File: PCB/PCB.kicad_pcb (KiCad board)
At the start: 4 copper layers, 21 x 51 mm, 33 parts, among them J1 USB_C_Receptacle_USB2.0_16P, J2 Conn_01x20, J3 Conn_01x20, SW1 SW_Push, U1 RP2040, U2 MCP1700x-330xxTT, U3 W25Q128JVS, Y1 Crystal_GND24

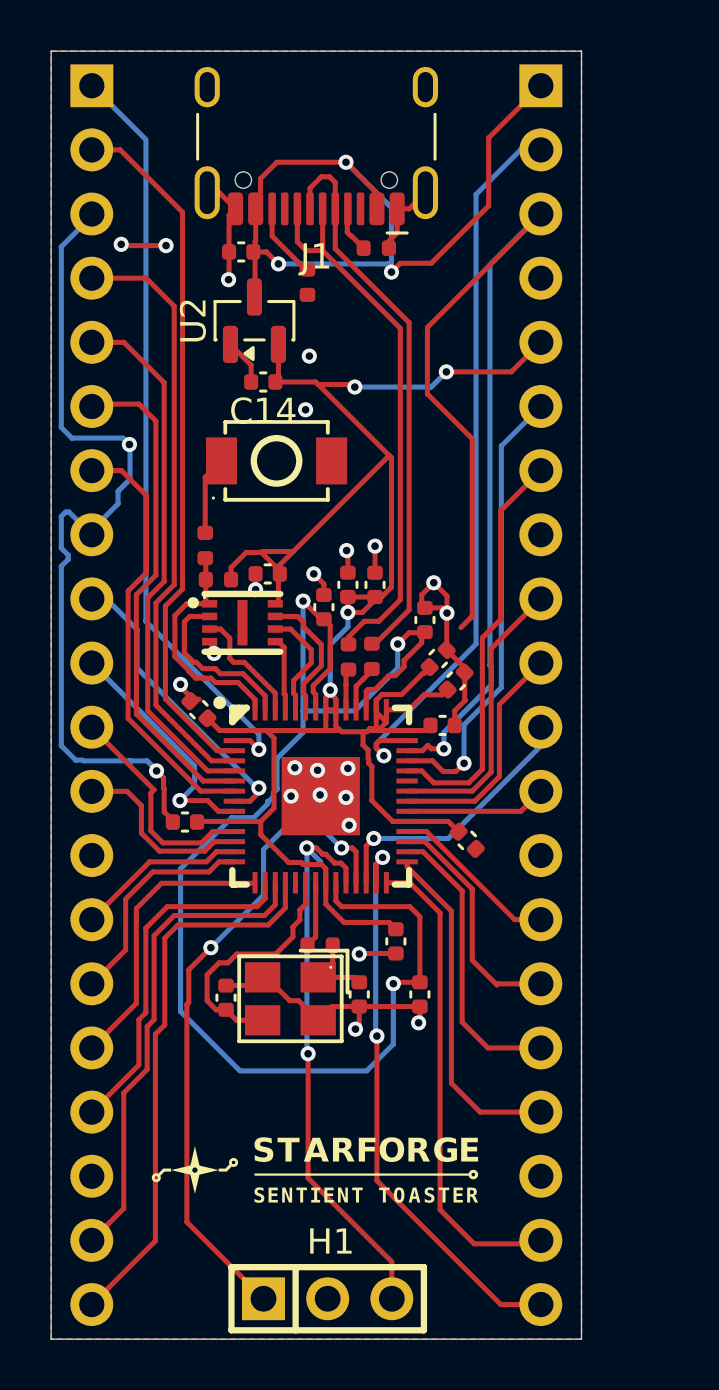
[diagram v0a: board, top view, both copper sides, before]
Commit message: finishing up project with BOM and FAB complete and clean.
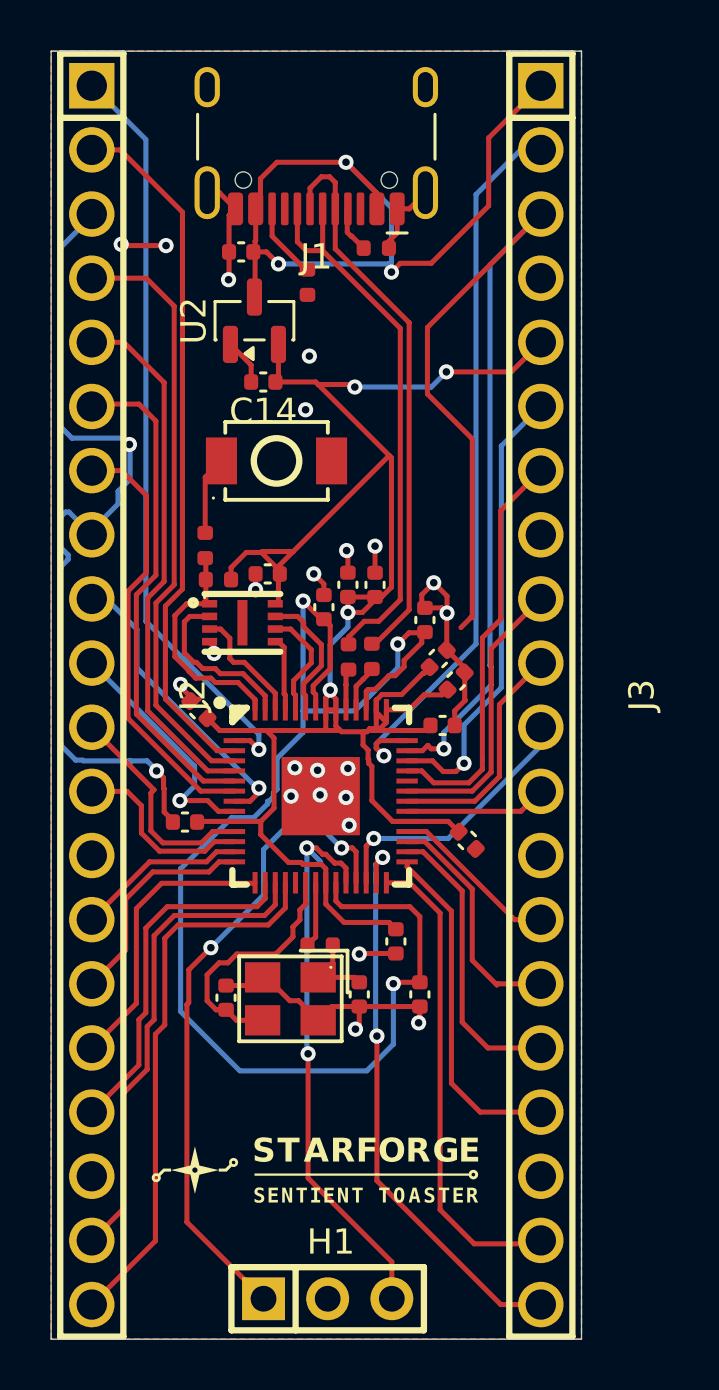
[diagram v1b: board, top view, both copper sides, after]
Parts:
- J2, J3: footprint Connector_PinHeader_2.54mm:PinHeader_1x20_P2.54mm_Vertical -> lcsc_footprints:C50981_HDR-TH_20P-P2_54-V-M-1; moved to F.Cu
- moved J2 24.1 mm to (123.1, 62.7), turned to -90 degrees
- moved J3 24.1 mm to (140.8, 62.7), turned to -90 degrees
